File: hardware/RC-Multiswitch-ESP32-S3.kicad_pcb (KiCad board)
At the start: 2 copper layers, 66.5 x 51.4 mm, 32 parts, among them CN1 UART A, CN2 5-12V, J1 Ausgaenge, J5 J5_UART B, J6 UART C, U1 ESP32-S3-Zero, U2 ULN2803A

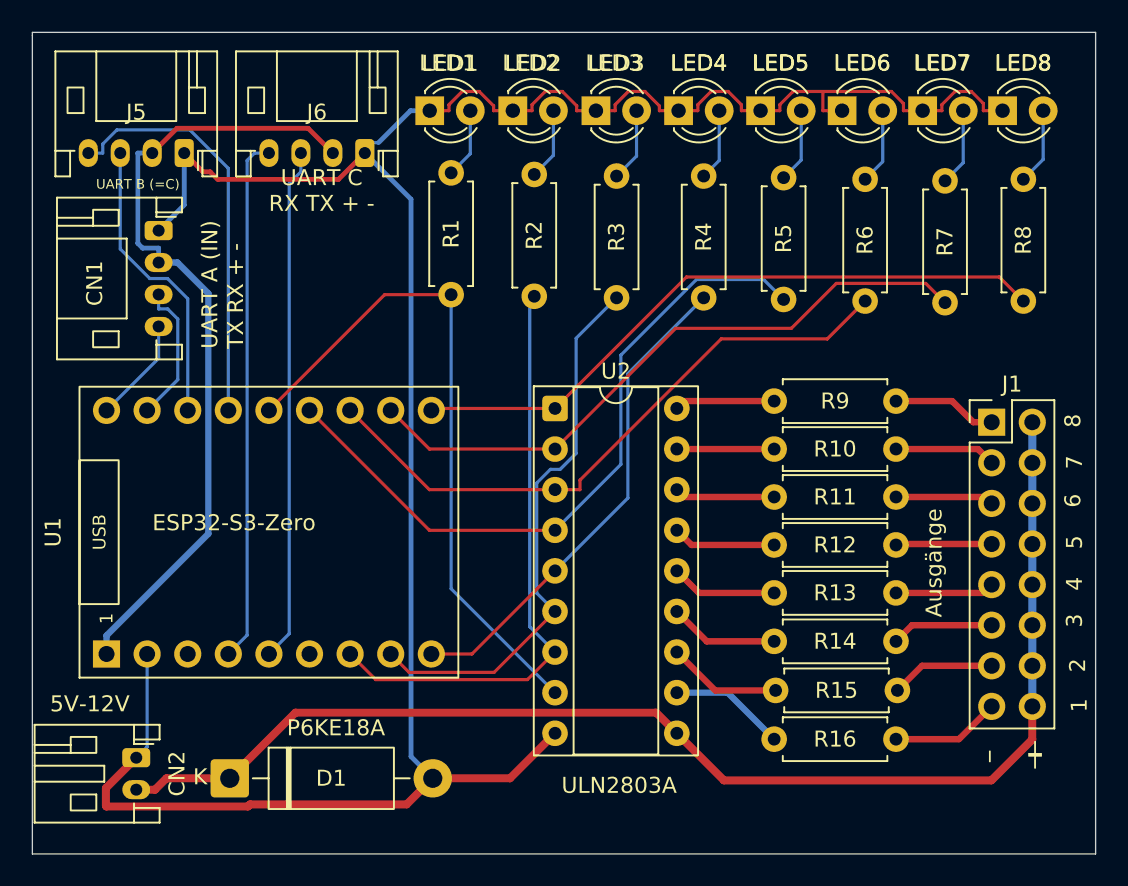
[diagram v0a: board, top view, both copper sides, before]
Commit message: PCB: Martins Stand 20.10. (nach Prüfung C3/S3)
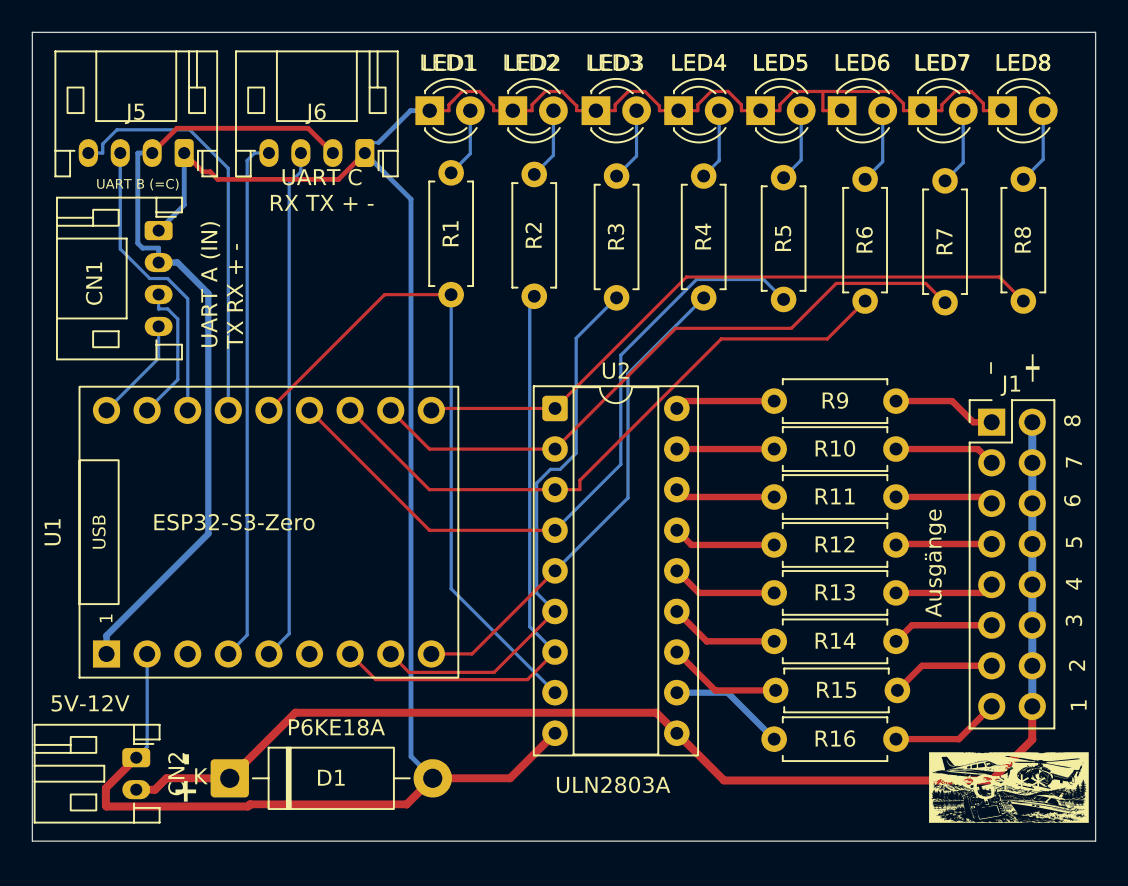
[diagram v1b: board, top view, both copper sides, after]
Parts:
- added G***: LOGO, LOGO, F.Cu at (184.9, 85.0)
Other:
- board size 66.5 x 51.4 mm -> 66.5 x 50.6 mm
- board text added: "+ -"
